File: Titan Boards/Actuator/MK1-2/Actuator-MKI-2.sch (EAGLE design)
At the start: 61 parts, among them Q1 MOSFET-NCH-AO3404A, Q10 MOSFET-NCH-AO3404A, Q11 MOSFET-NCH-AO3404A, Q12 MOSFET-NCH-AO3404A, Q13 MOSFET-NCH-AO3404A, Q14 MOSFET-NCH-AO3404A, Q15 MOSFET-NCH-AO3404A, Q16 MOSFET-NCH-AO3404A, Q17 MOSFET-NCH-AO3404A, Q18 FDD4141TO252, Q2 MOSFET-NCH-AO3404A, Q3 MOSFET-NCH-AO3404A, Q4 MOSFET-NCH-AO3404A, Q5 MOSFET-NCH-AO3404A, Q6 FDD4141TO252, Q7 MOSFET-NCH-AO3404A, Q8 MOSFET-NCH-AO3404A, Q9 MOSFET-NCH-AO3404A, U1 DRV8816PWPR

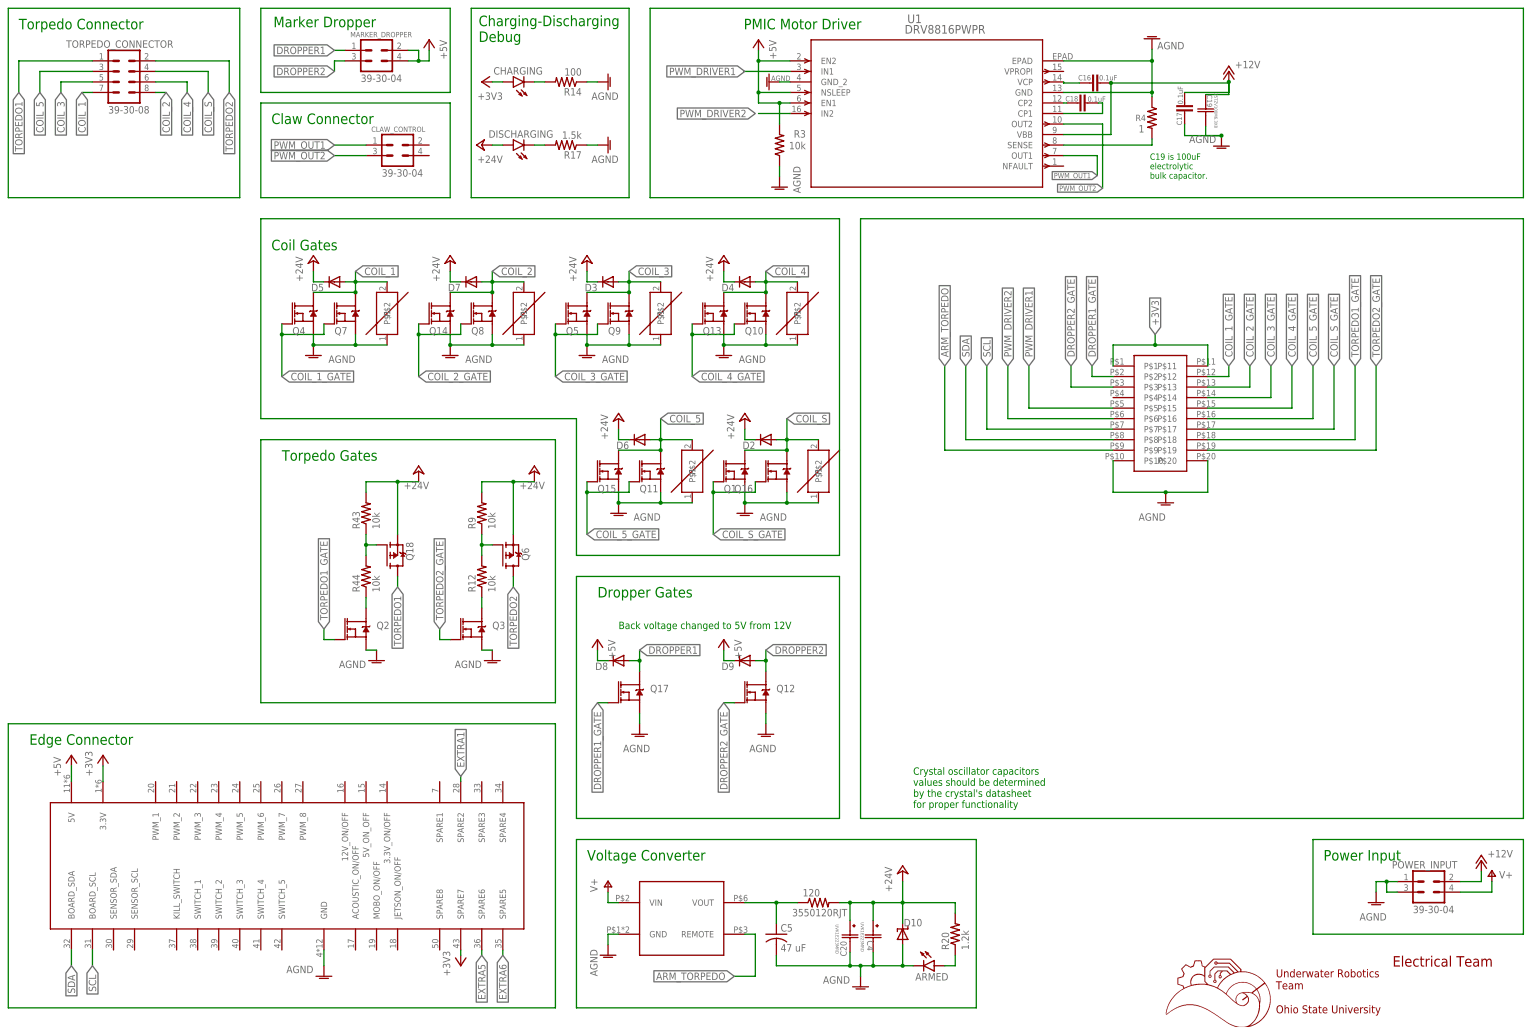
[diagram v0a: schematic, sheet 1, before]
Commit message: Tempest Actuator MK1-2 Updates
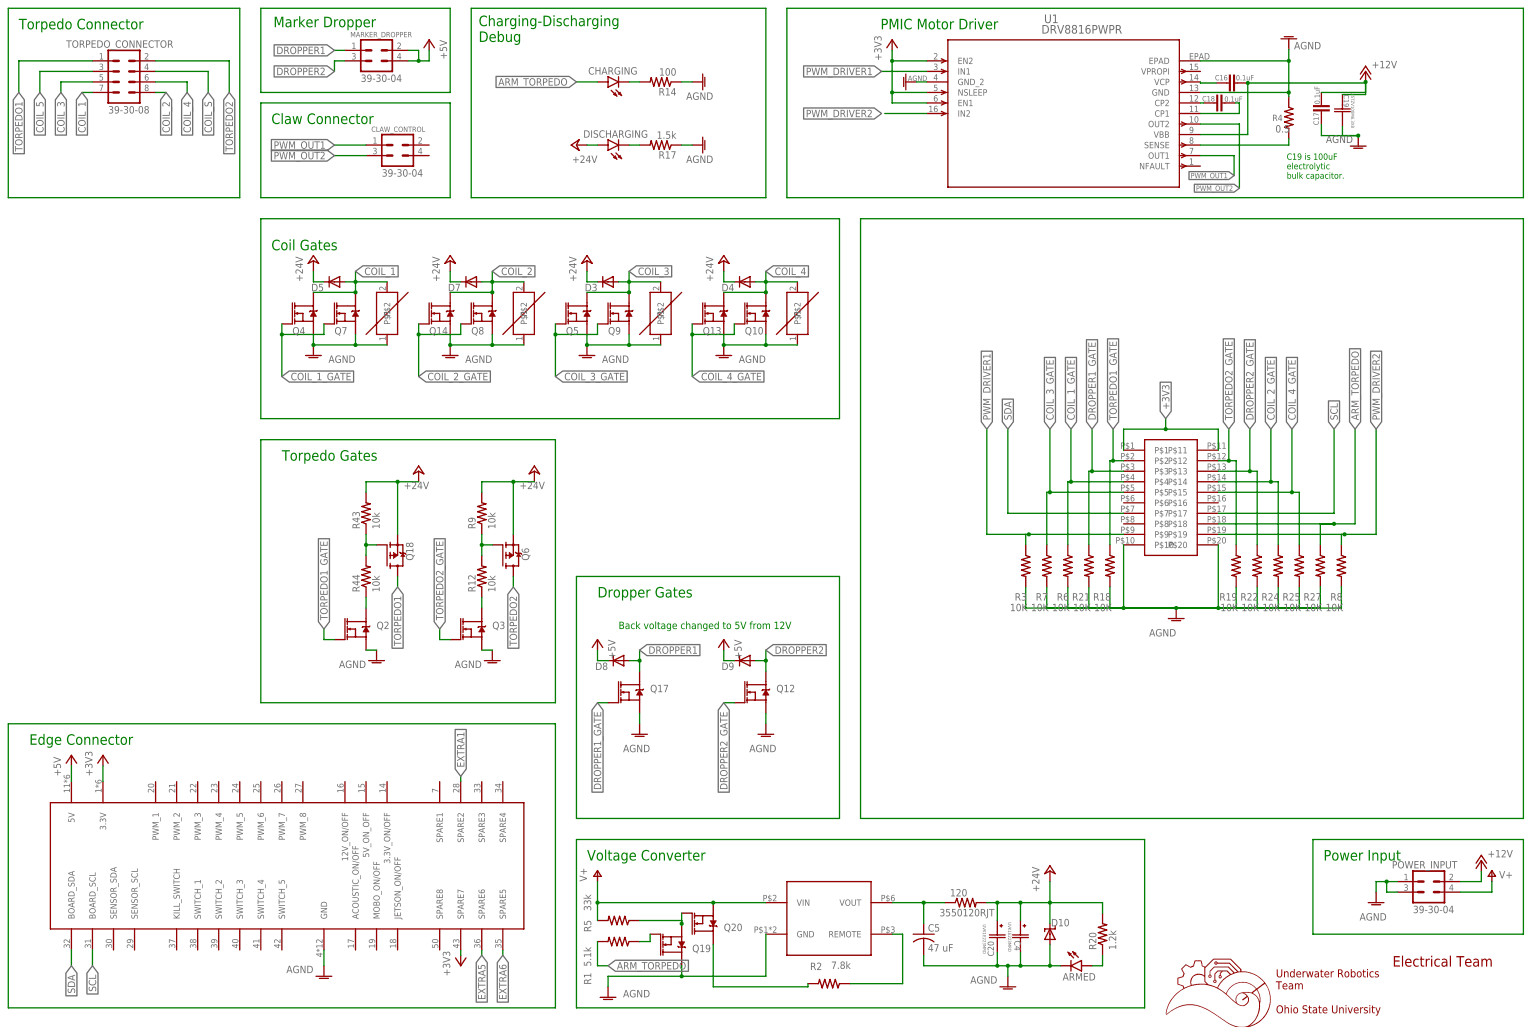
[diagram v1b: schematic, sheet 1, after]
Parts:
- removed D2, D6: (no value), diode:DIODE-SMB
- removed Q1, Q11, Q15, Q16: MOSFET-NCH-AO3404A, SparkFun-DiscreteSemi:MOSFET-NCH-AO3404A
- removed U$2, U$3: ERZ-VF2M270ERZ-VF2M270, ERZ-VF2M270:ERZ-VF2M270ERZ-VF2M270
- added Q19, Q20: MOSFET-NCH-AO3404A, SparkFun-DiscreteSemi:MOSFET-NCH-AO3404A
- added R1: 5.1k, resistor:R-US_R0603
- added R18, R19, R21, R22, R24, R25, R27, R6, R7, R8: 10K, resistor:R-US_R0603
- added R2: 7.8k, resistor:R-US_R0603
- added R5: 33k, resistor:R-US_R0603
- R3: value 10k -> 10K
- R4: value 1 -> 0.5
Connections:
- removed net COIL_5_GATE: Q11.G, Q15.G, U$9.P$16
- removed net COIL_S_GATE: Q1.G, Q16.G, U$9.P$17
- new net N$3: R2.1, U$6.REMOTE
- new net N$5: Q19.G, R1.1
- new net N$6: Q19.S, Q20.G, R5.1
- new net N$7: Q20.D, R2.2
- net +24V: no longer D2.C, D6.C
- net +3V3: now also U1.EN1, U1.EN2, U1.NSLEEP; no longer CHARGING.A
- net +5V: no longer R3.2, U1.EN1, U1.EN2, U1.NSLEEP
- net AGND: now also Q19.D, R18.2, R19.2, R21.2, R22.2, R24.2, R25.2, R27.2, R3.2, R6.2, R7.2, R8.2; no longer Q1.S, Q11.S, Q15.S, Q16.S, R3.1, U$2.P$1, U$3.P$1
- net ARM_TORPEDO: now also CHARGING.A, R1.2, R27.1, U$9.P$18; no longer U$6.REMOTE, U$9.P$9
- net COIL_1_GATE: now also R6.1, U$9.P$4; no longer U$9.P$12
- net COIL_2_GATE: now also R24.1, U$9.P$14; no longer U$9.P$13
- net COIL_3_GATE: now also R7.1, U$9.P$5; no longer U$9.P$14
- net COIL_4_GATE: now also R25.1
- net COIL_5: no longer D6.A, Q11.D, Q15.D, U$3.P$2
- net COIL_S: no longer D2.A, Q1.D, Q16.D, U$2.P$2
- net DROPPER1_GATE: now also R21.1, U$9.P$3; no longer U$9.P$2
- net DROPPER2_GATE: now also R22.1, U$9.P$13; no longer U$9.P$3
- net PWM_DRIVER1: now also R3.1, U$9.P$9; no longer U$9.P$5
- net PWM_DRIVER2: now also R8.1, U$9.P$19; no longer U$9.P$6
- net SCL: now also U$9.P$17; no longer U$9.P$7
- net SDA: now also U$9.P$7; no longer U$9.P$8
- net TORPEDO1_GATE: now also R18.1, U$9.P$2; no longer U$9.P$18
- net TORPEDO2_GATE: now also R19.1, U$9.P$12; no longer U$9.P$19
- net V+: now also Q20.S, R5.2
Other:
- note removed: "Crystal oscillator capacitors values should be determined by the crystal's datasheet for proper functionality"
- moved on the sheet: 120, ARMED, C16, C17, C18, C19, C20, C4, C5, CHARGING, D10, DISCHARGING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
